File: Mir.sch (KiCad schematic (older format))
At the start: 34 parts, among them SW1 SW_PUSH, U1 ATMEGA32U2-AU, U2 PRTR5V0U2X, Y1 16MHz

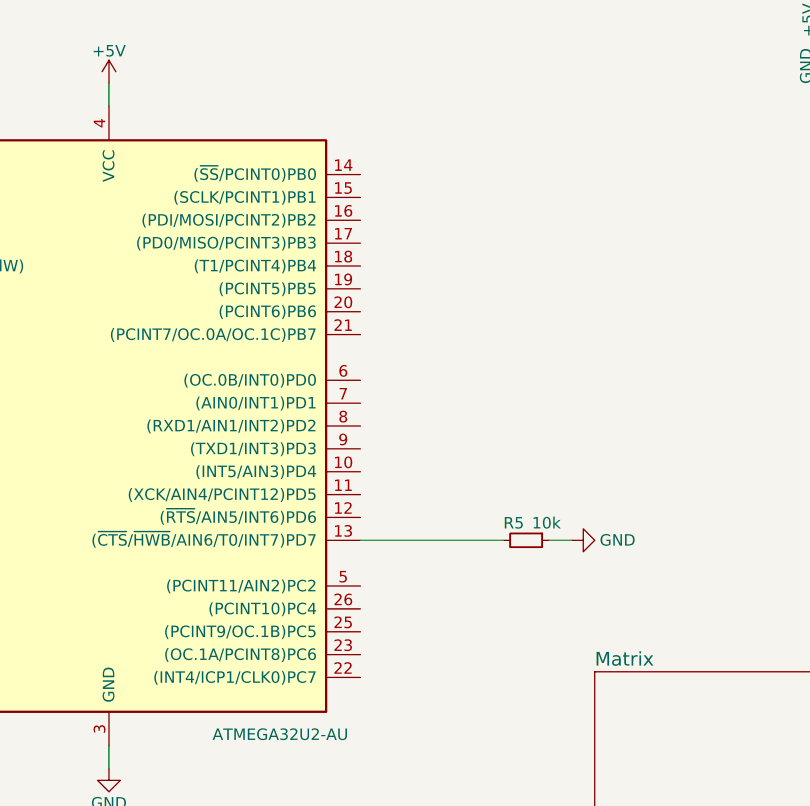
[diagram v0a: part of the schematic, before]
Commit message: Finish routing
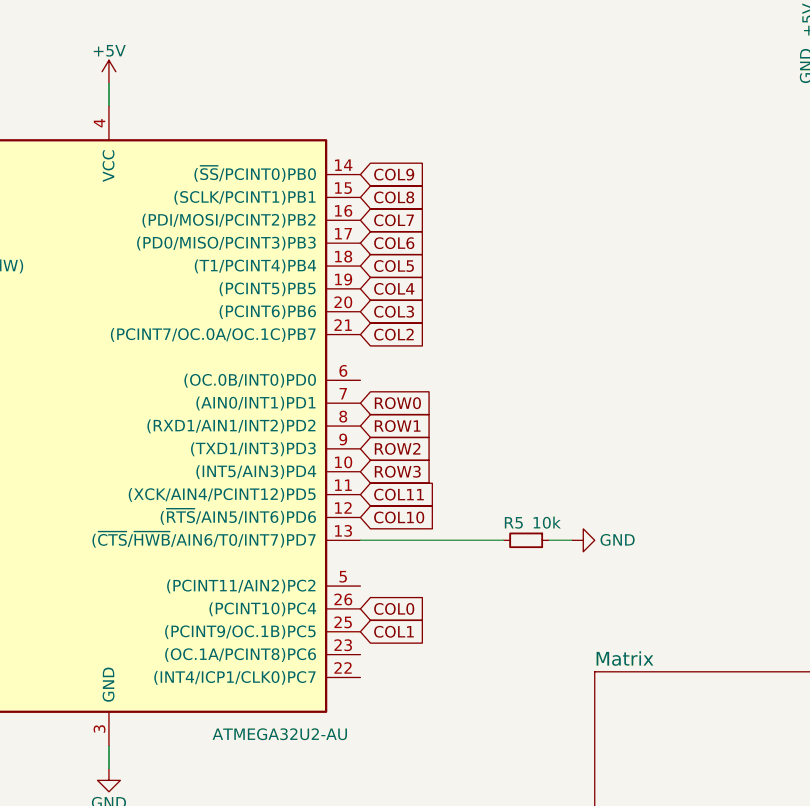
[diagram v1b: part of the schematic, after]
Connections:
- net labels added: COL0, COL1, COL10, COL11, COL2, COL3, COL4, COL5, COL6, COL7, COL8, COL9, ROW0, ROW1, ROW2, ROW3
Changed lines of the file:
@@
 $EndComp
 Connection ~ 2100 6700
+Text GLabel 4250 3800 2    50   Input ~ 0
+COL0
+Text GLabel 4250 3900 2    50   Input ~ 0
+COL1
+Text GLabel 4250 2600 2    50   Input ~ 0
+COL2
+Text GLabel 4250 2500 2    50   Input ~ 0
+COL3
+Text GLabel 4250 2400 2    50   Input ~ 0
+COL4
+Text GLabel 4250 2300 2    50   Input ~ 0
+COL5
+Text GLabel 4250 2200 2    50   Input ~ 0
+COL6
+Text GLabel 4250 2100 2    50   Input ~ 0
+COL7
+Text GLabel 4250 2000 2    50   Input ~ 0
+COL8
+Text GLabel 4250 1900 2    50   Input ~ 0
+COL9
+Text GLabel 4250 3400 2    50   Input ~ 0
+COL10
+Text GLabel 4250 3300 2    50   Input ~ 0
+COL11
+Text GLabel 4250 3200 2    50   Input ~ 0
+ROW3
+Text GLabel 4250 3100 2    50   Input ~ 0
+ROW2
+Text GLabel 4250 3000 2    50   Input ~ 0
+ROW1
+Text GLabel 4250 2900 2    50   Input ~ 0
+ROW0
 $EndSCHEMATC
